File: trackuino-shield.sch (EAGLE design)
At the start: 20 parts, among them IC2 AP1117, J5 J5MM, M2 HX1, U1 LM60 int, X1 BU-SMA-V, X2 Vin, X3 LM60 ext, X4 Buzzer

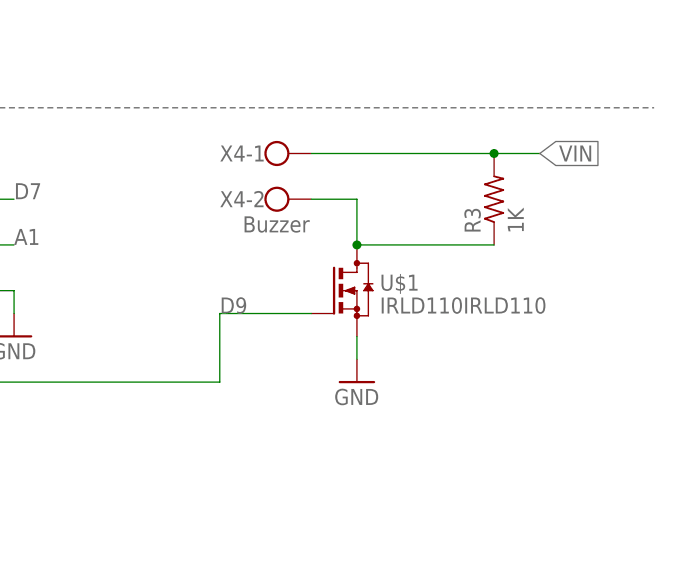
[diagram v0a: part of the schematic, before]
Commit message: Minor routing change
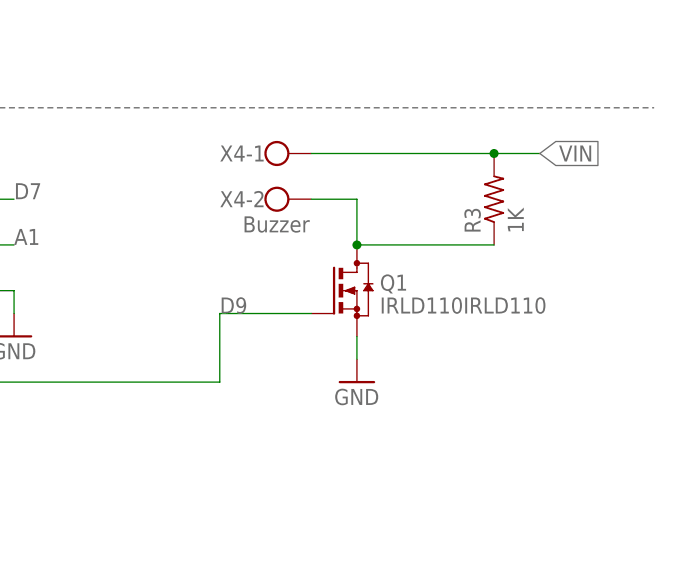
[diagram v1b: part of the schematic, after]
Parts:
- renumbered U$1 to Q1
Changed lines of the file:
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@@
 <part name="IC2" library="First" deviceset="AP1117" device=""/>
 <part name="GPS" library="trackuino" deviceset="VENUS638FLPX" device=""/>
-<part name="U$1" library="First" deviceset="IRLD110" device="IRLD110"/>
+<part name="Q1" library="First" deviceset="IRLD110" device="IRLD110"/>
 </parts>
 <sheets>
@@
 <instance part="IC2" gate="G$1" x="30.48" y="154.94"/>
 <instance part="GPS" gate="G$1" x="106.68" y="93.98"/>
-<instance part="U$1" gate="G$1" x="231.14" y="50.8"/>
+<instance part="Q1" gate="G$1" x="231.14" y="50.8"/>
 </instances>
 <busses>
@@
 <wire x1="231.14" y1="43.18" x2="231.14" y2="45.72" width="0.1524" layer="91"/>
 <pinref part="GND14" gate="1" pin="GND"/>
-<pinref part="U$1" gate="G$1" pin="S"/>
+<pinref part="Q1" gate="G$1" pin="S"/>
 </segment>
 <segment>
@@
 <wire x1="30.48" y1="40.64" x2="215.9" y2="40.64" width="0.1524" layer="91"/>
 <wire x1="215.9" y1="40.64" x2="215.9" y2="48.26" width="0.1524" layer="91"/>
-<pinref part="U$1" gate="G$1" pin="G"/>
+<pinref part="Q1" gate="G$1" pin="G"/>
 </segment>
 </net>
@@
 <pinref part="X4" gate="-2" pin="KL"/>
 <pinref part="R3" gate="G$1" pin="1"/>
-<pinref part="U$1" gate="G$1" pin="D"/>
+<pinref part="Q1" gate="G$1" pin="D"/>
 <junction x="231.14" y="55.88"/>
 </segment>
